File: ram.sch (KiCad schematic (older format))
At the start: 2 parts, among them U2 AS6C4008

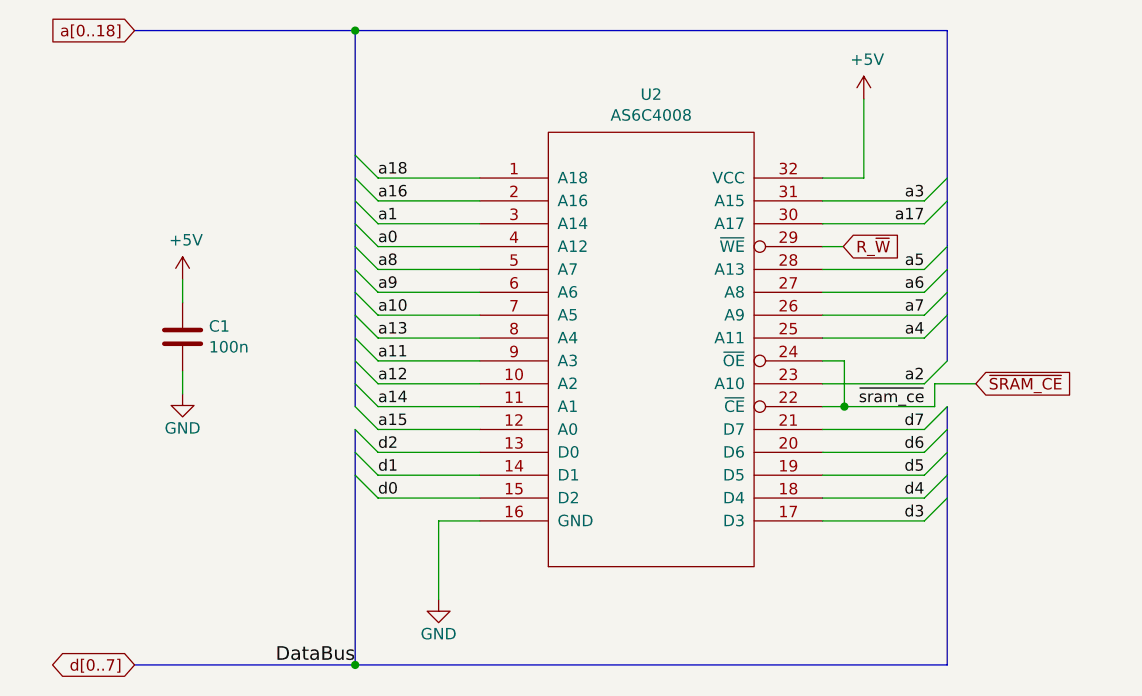
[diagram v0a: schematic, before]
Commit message: More rerouting
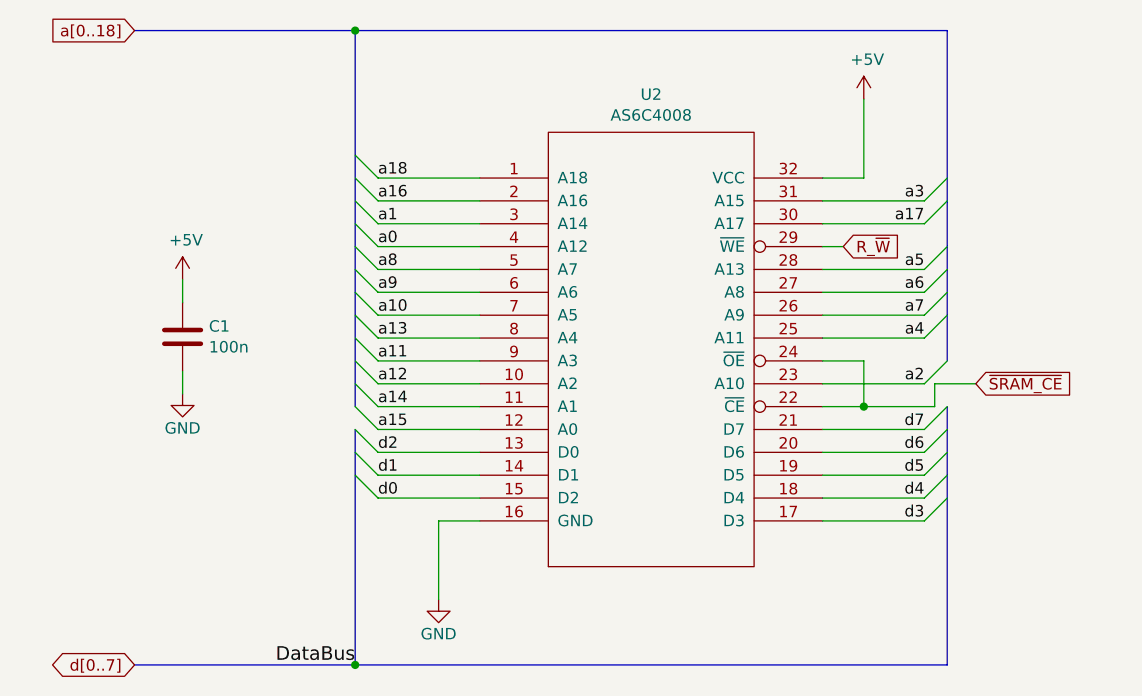
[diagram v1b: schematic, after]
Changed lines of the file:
@@
 Text GLabel 6275 2895 0    50   Input ~ 0
 a[0..18]
-Text Label 9730 4540 2    50   ~ 0
-~sram_ce
-Wire Wire Line
-	9285 4340 9380 4340
-Wire Wire Line
-	9380 4340 9380 4540
-Connection ~ 9380 4540
-Wire Wire Line
-	9380 4540 9285 4540
 Text GLabel 9955 4440 2    50   Input ~ 0
 ~SRAM_CE
@@
 Wire Wire Line
 	9775 4440 9955 4440
-Wire Wire Line
-	9380 4540 9775 4540
 Text Label 9730 4040 2    50   ~ 0
 a6
@@
 Text Label 9730 4640 2    50   ~ 0
 d7
+Wire Wire Line
+	9285 4540 9465 4540
+Wire Wire Line
+	9285 4340 9465 4340
+Wire Wire Line
+	9465 4340 9465 4540
 Wire Bus Line
 	7240 4640 7240 5670
@@
 Wire Bus Line
 	7240 2895 7240 4540
+Connection ~ 9465 4540
+Wire Wire Line
+	9465 4540 9775 4540
 $EndSCHEMATC
